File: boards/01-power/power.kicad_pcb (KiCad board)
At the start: 8 copper layers, 50 x 50 mm, 44 parts, among them J1 CONN_DF40_100P_F, J2 USB_C_Receptacle_USB2.0_16P, P1 MAG_RB1_125BAG1A, SW1 SW_BOOT, SW2 SW_BOOT, SW3 SW_BOOT, U1 USBLC6-2P6, U2 AP63203WU, U3 STM32F405RGTx, Y1 16Mhz

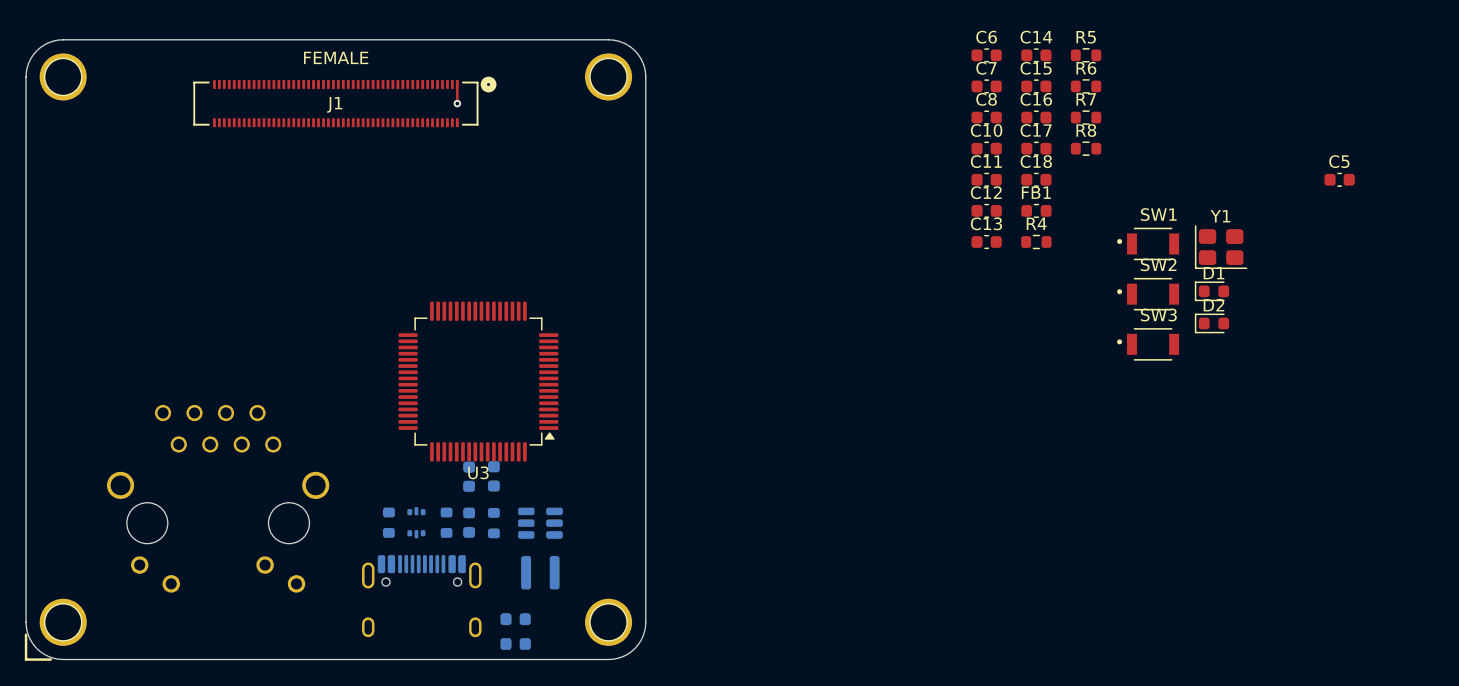
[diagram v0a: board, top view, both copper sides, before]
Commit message: wip: 3.3v
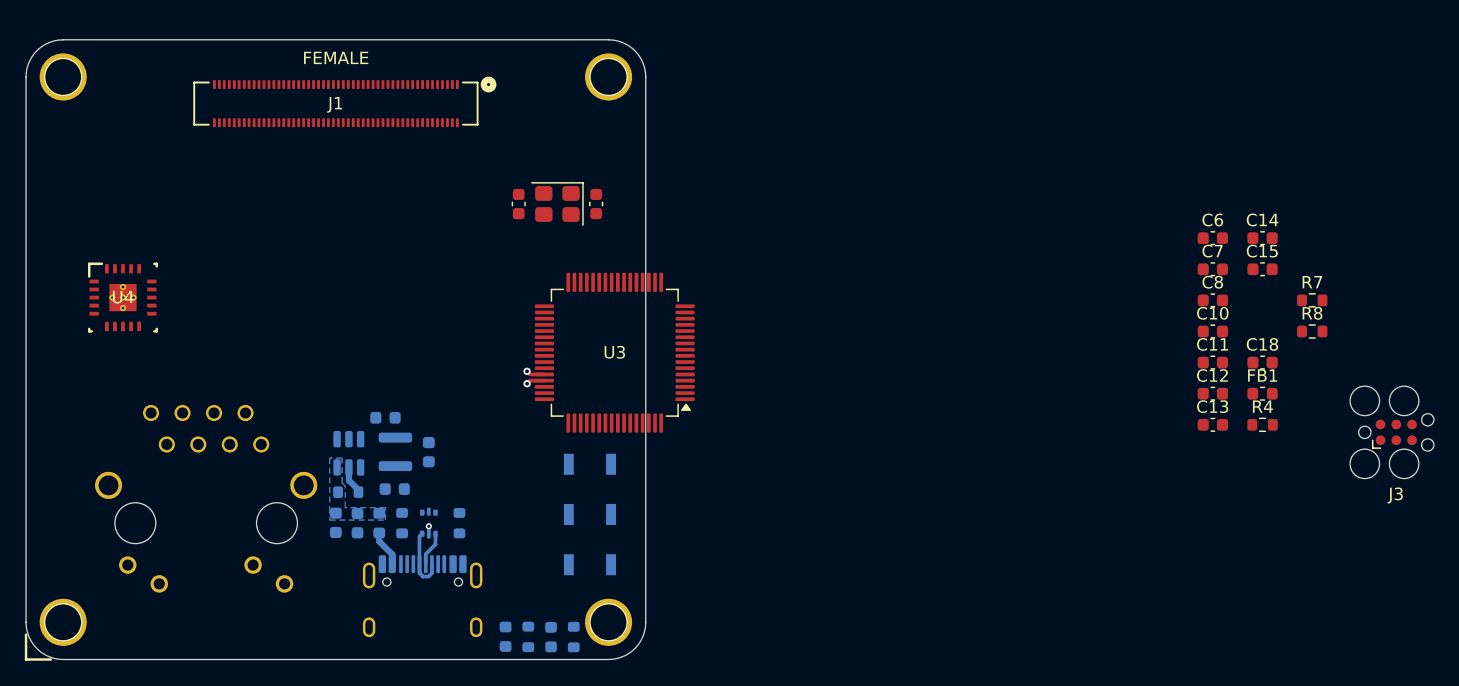
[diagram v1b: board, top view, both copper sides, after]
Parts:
- removed SW1: SW_BOOT, Woki:SW_B3U_1000P
- added BOOT: SW_BOOT, Woki:SW_B3U_1000P, B.Cu at (95.5, 84.2)
- added J3: TC2030, Connector:Tag-Connect_TC2030-IDC-FP_2x03_P1.27mm_Vertical, F.Cu at (160.6, 81.7)
- added U4: PMIC_TPS2372_4RGWR, Woki:PMIC_TPS2372_4RGWR, F.Cu at (57.8, 70.8)
- C5, D1, D2, R5, R6, SW2, SW3: moved to B.Cu
- moved C5 79.3 mm to (79.0, 80.5)
- moved R6 63.2 mm to (90.5, 98.2), turned to 90 degrees
- moved R5 62.5 mm to (94.2, 98.2), turned to 90 degrees
- moved D2 62.5 mm to (88.7, 98.2), turned to 90 degrees
- moved D1 60.3 mm to (92.4, 98.2), turned to 90 degrees
- moved Y1 53.7 mm to (92.9, 63.2), turned to 180 degrees
- moved SW2 48.8 mm to (95.5, 88.3), turned to 180 degrees
- moved SW3 48.8 mm to (95.5, 92.3), turned to 180 degrees
- moved C17 42.0 mm to (89.8, 63.2), turned to 90 degrees
- moved C16 36.2 mm to (96.0, 63.2), turned to -90 degrees
- moved C12 23.5 mm to (145.8, 78.6)
- moved C8 23.5 mm to (145.8, 71.0)
- moved FB1 23.5 mm to (149.8, 78.6)
- moved R7 23.5 mm to (153.8, 71.0)
- moved C10 23.5 mm to (145.8, 73.5)
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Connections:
- net Net-(U3-NRST) renamed /STM32/~{STM_RESET}
- D1 pad 1: GND -> Net-(D1-K)
- D1 pad 2: Net-(D1-A) -> /STM32/LED_STATUS
- D2 pad 1: GND -> Net-(D2-K)
- D2 pad 2: Net-(D2-A) -> /STM32/LED_ERROR
- R5 pad 1: /STM32/LED_STATUS -> Net-(D1-K)
- R5 pad 2: Net-(D1-A) -> GND
- R6 pad 1: /STM32/LED_ERROR -> Net-(D2-K)
- R6 pad 2: Net-(D2-A) -> GND
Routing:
- net /USB/D-: track 0.00 -> 5.22 mm
- net Net-(U1-VBUS): track 0.00 -> 2.96 mm
- net /USB/D+: track 0.00 -> 2.78 mm
- net /USB/~{EN}: track 0.00 -> 2.32 mm
- net +12V_BULK: track 1.54 -> 0.00 mm, vias 1 -> 0
- net /STM32/USB_D-: track 0.00 -> 1.50 mm, vias 0 -> 1
- net /STM32/USB_D+: track 0.00 -> 1.50 mm, vias 0 -> 1
- net GND: track 0.00 -> 0.67 mm, vias 0 -> 1
- added copper zone on B.Cu, net /USB/VBUS

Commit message: wip: buck (plan layout rough)
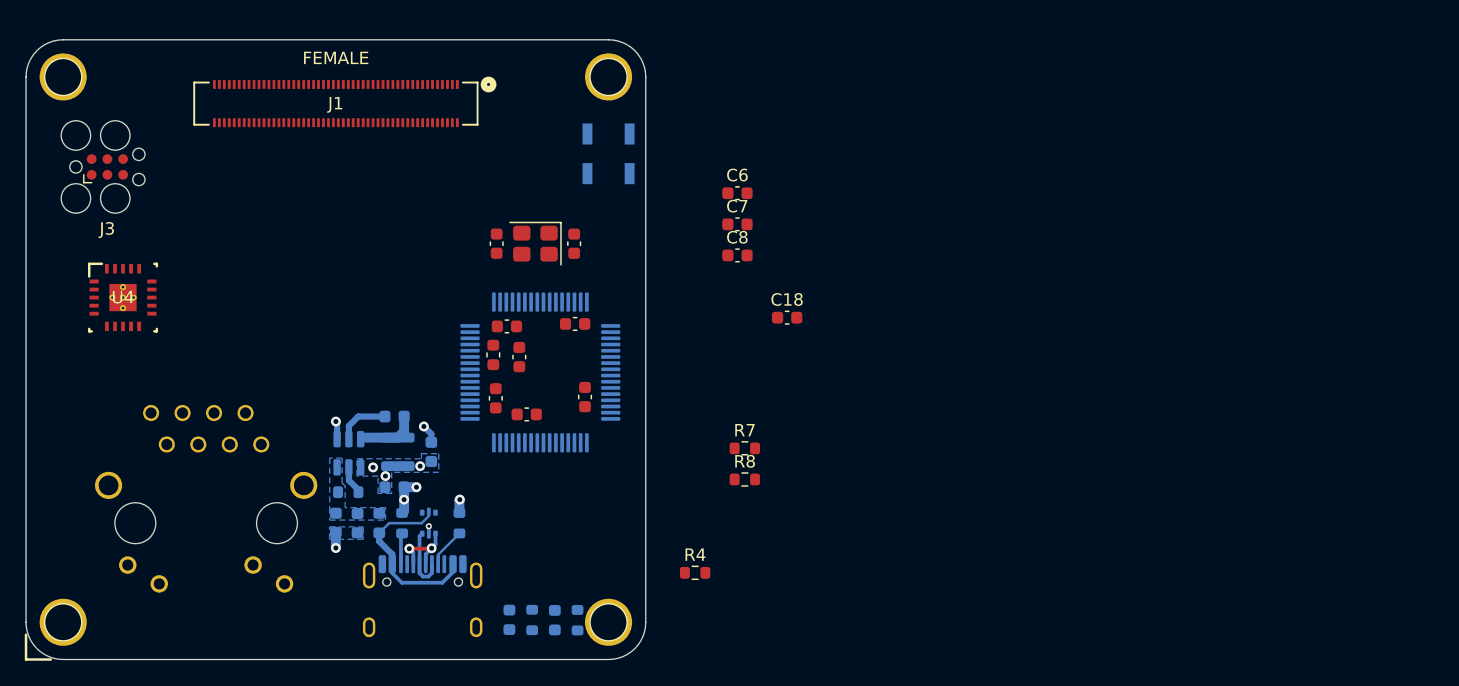
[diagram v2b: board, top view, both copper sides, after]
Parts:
- removed BOOT, SW3: SW_BOOT, Woki:SW_B3U_1000P
- added SW1: SW_BOOT, Woki:SW_B3U_1000P, B.Cu at (97.0, 60.8)
- U3: moved to B.Cu
- moved J3 106.2 mm to (56.6, 60.3)
- moved FB1 62.1 mm to (87.7, 75.4), turned to 90 degrees
- moved C15 60.4 mm to (89.8, 75.6), turned to 90 degrees
- moved C12 57.9 mm to (87.9, 78.9), turned to 90 degrees
- moved C13 57.5 mm to (88.8, 73.1), turned to 180 degrees
- moved C14 55.9 mm to (94.3, 72.9), turned to 180 degrees
- moved C11 55.5 mm to (90.4, 80.2)
- moved C10 50.9 mm to (95.1, 78.8), turned to 90 degrees
- moved R7 47.3 mm to (108.0, 83.0)
- moved R8 47.3 mm to (108.0, 85.5)
- moved R4 47.3 mm to (104.0, 93.0)
- moved C18 38.5 mm to (111.4, 72.4)
- moved C6 38.5 mm to (107.4, 62.4)
- moved C7 38.5 mm to (107.4, 64.9)
- moved C8 38.5 mm to (107.4, 67.4)
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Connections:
- U3 pad 11: /STM32/USR_BTN2 -> unconnected-(U3-PC3-Pad11)
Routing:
- net Net-(U1-VBUS): track 2.96 -> 14.8 mm
- net GND: track 0.67 -> 9.14 mm, vias 1 -> 7
- net Net-(U2-BST): track 0.00 -> 4.78 mm
- net Net-(U2-SW): track 0.00 -> 4.29 mm
- net Net-(J2-CC1): track 0.00 -> 3.19 mm
- net /USB/D+: track 2.78 -> 5.93 mm, vias 0 -> 2
- net Net-(J2-CC2): track 0.00 -> 2.52 mm
- net /STM32/USB_D-: track 1.50 -> 0.00 mm, vias 1 -> 0
- net /STM32/USB_D+: track 1.50 -> 0.00 mm, vias 1 -> 0
- net +3.3V: vias 0 -> 3
- added copper zone on B.Cu, net +3.3V
- added copper zone on B.Cu, net GND
